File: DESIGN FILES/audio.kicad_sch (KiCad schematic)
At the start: 22 parts, among them J501 PJ-342B-TX-SMT, J502 PJ-342B-TX-SMT, J503 PJ-342B-TX-SMT, U501 WM8978CGEFL_RV

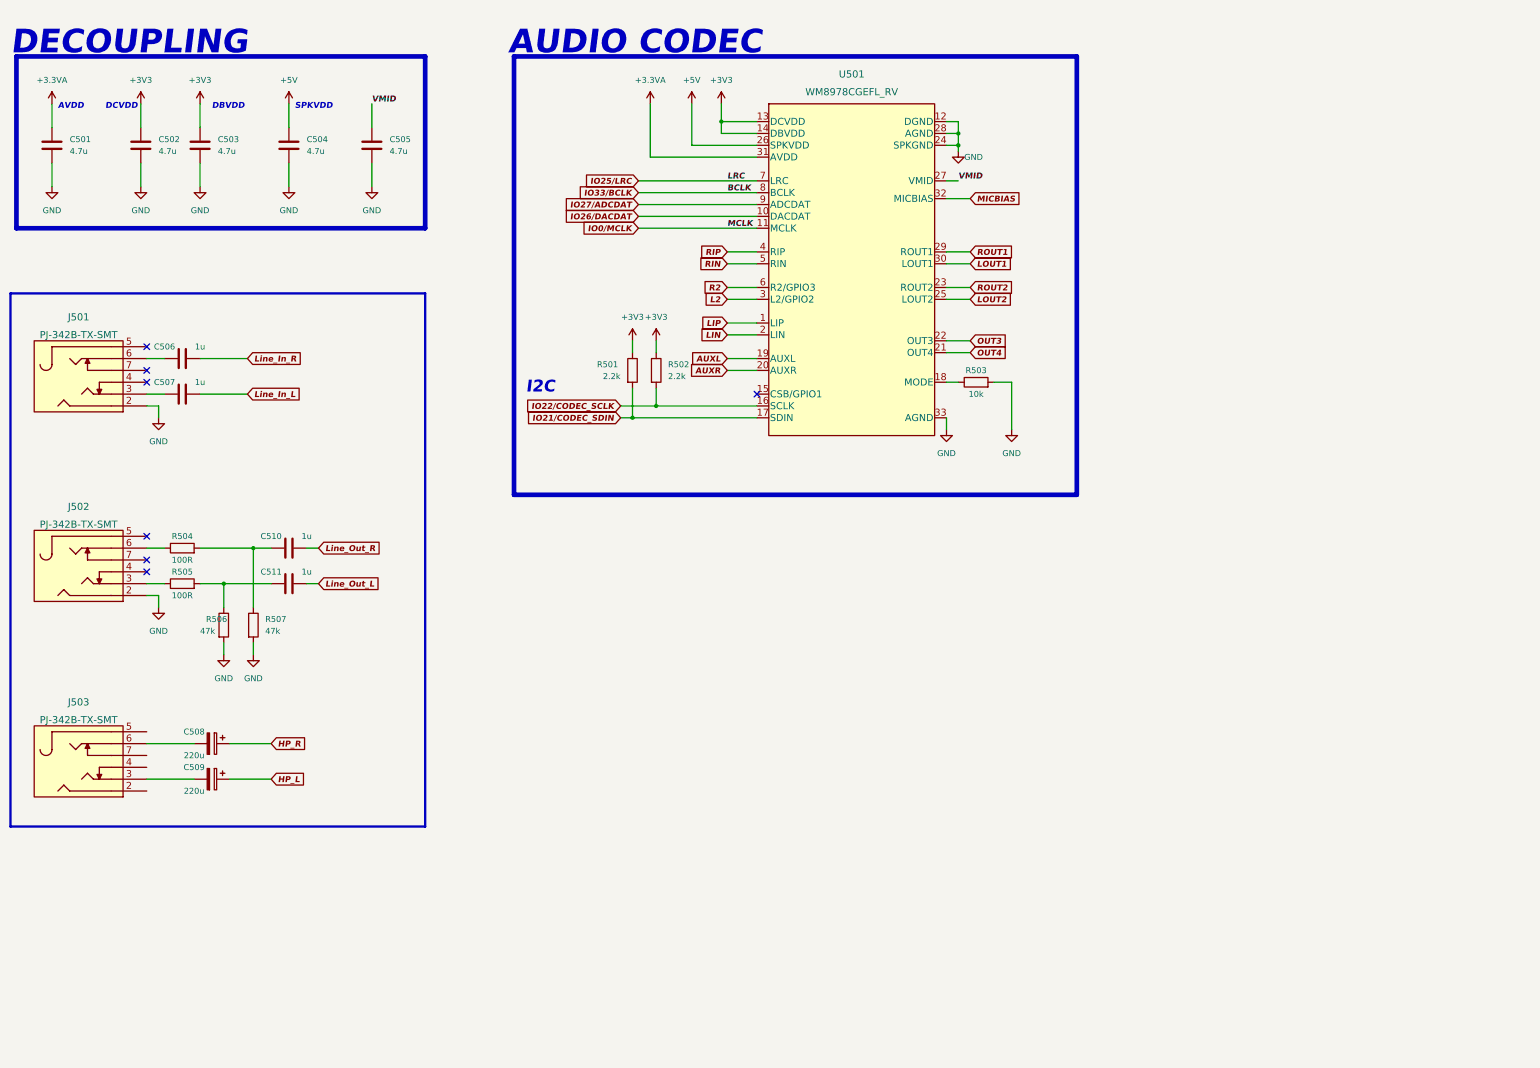
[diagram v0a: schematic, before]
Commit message: updates
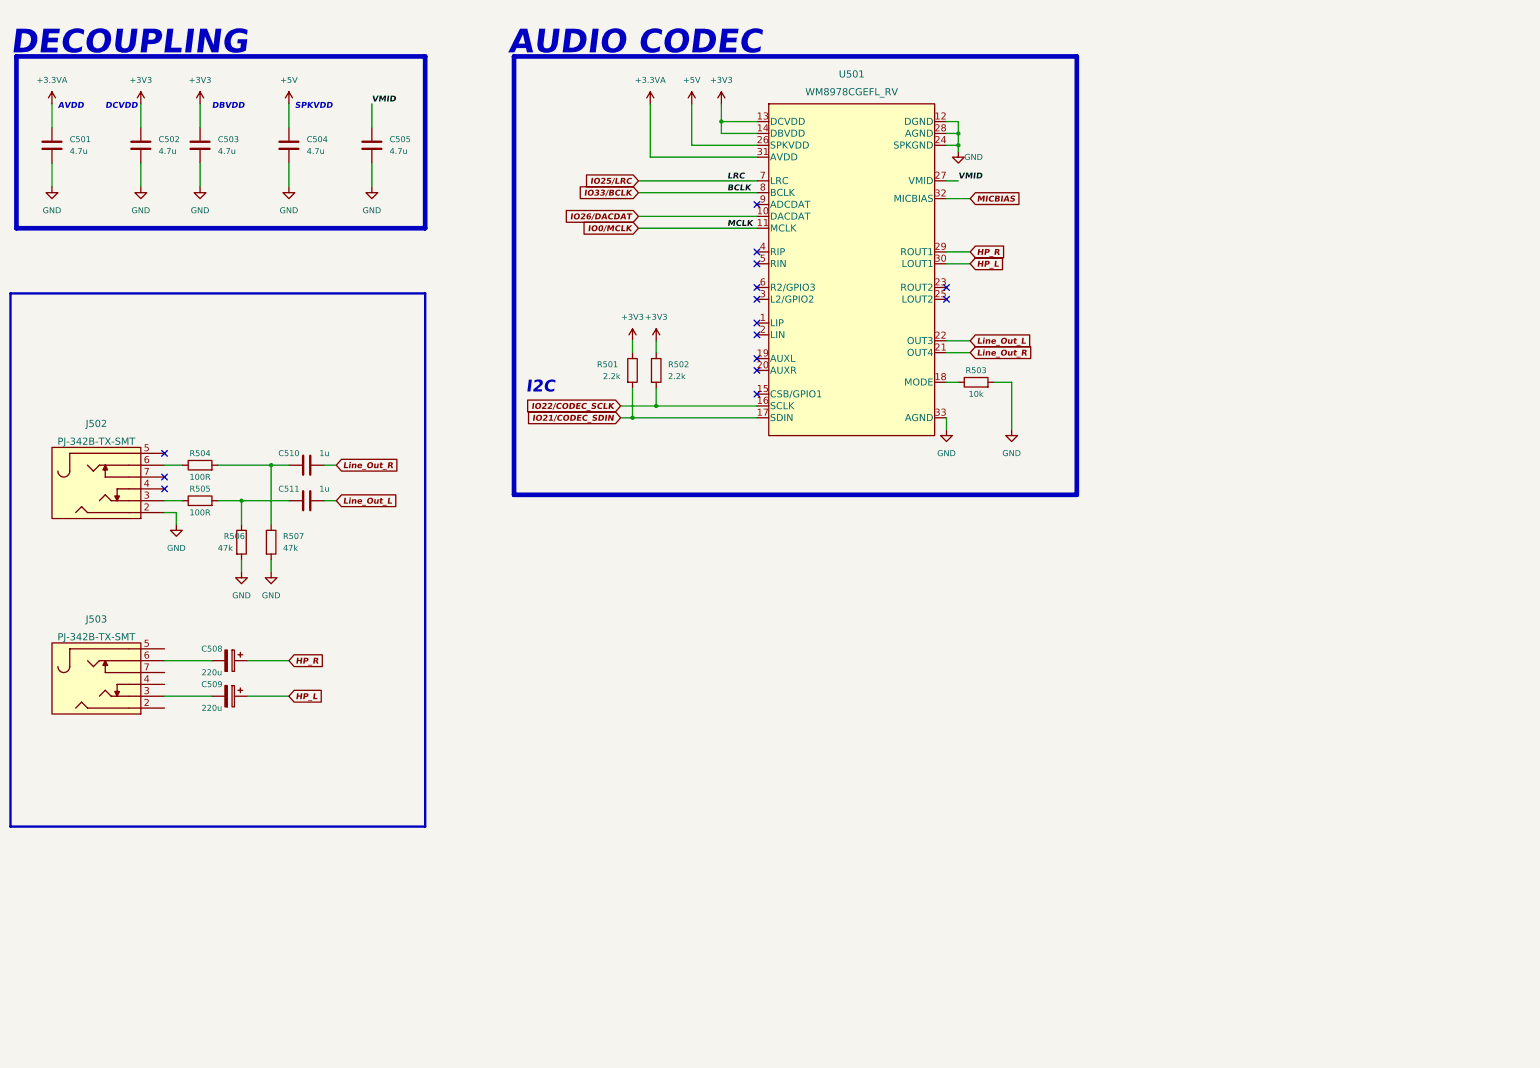
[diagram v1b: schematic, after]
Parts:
- removed C506, C507: 1u, MY CAPACITOR LIBRARY:CL10A105KB8NNNC_0603, symbol MY CAPACITOR LIBRARY:CL10A105KB8NNNC
- removed J501: PJ-342B-TX-SMT, MY CONNECTOR LIBRARY:PJ-342B-TX-SMT, symbol MY CONNECTOR LIBRARY:PJ-342B-TX-SMT
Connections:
- net LOUT1 is gone; now on net HP_L: U501.30 (LOUT1)
- net OUT3 is gone; now on net Line_Out_L: U501.22 (OUT3)
- net OUT4 is gone; now on net Line_Out_R: U501.21 (OUT4)
- net ROUT1 is gone; now on net HP_R: U501.29 (ROUT1)
- net AUXL: no longer names the net of U501.19 (AUXL)
- net AUXR: no longer names the net of U501.20 (AUXR)
- net IO27/ADCDAT: no longer names the net of U501.9 (ADCDAT)
- net L2: no longer names the net of U501.3 (L2/GPIO2)
- net LIN: no longer names the net of U501.2 (LIN)
- net LIP: no longer names the net of U501.1 (LIP)
- net LOUT2: no longer names the net of U501.25 (LOUT2)
- net R2: no longer names the net of U501.6 (R2/GPIO3)
- net RIN: no longer names the net of U501.5 (RIN)
- net RIP: no longer names the net of U501.4 (RIP)
- net ROUT2: no longer names the net of U501.23 (ROUT2)
- no-connect marks 7 -> 15
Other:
- moved on the sheet: C508, C509, C510, C511, J502, J503, R504, R505, R506, R507

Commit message: updates
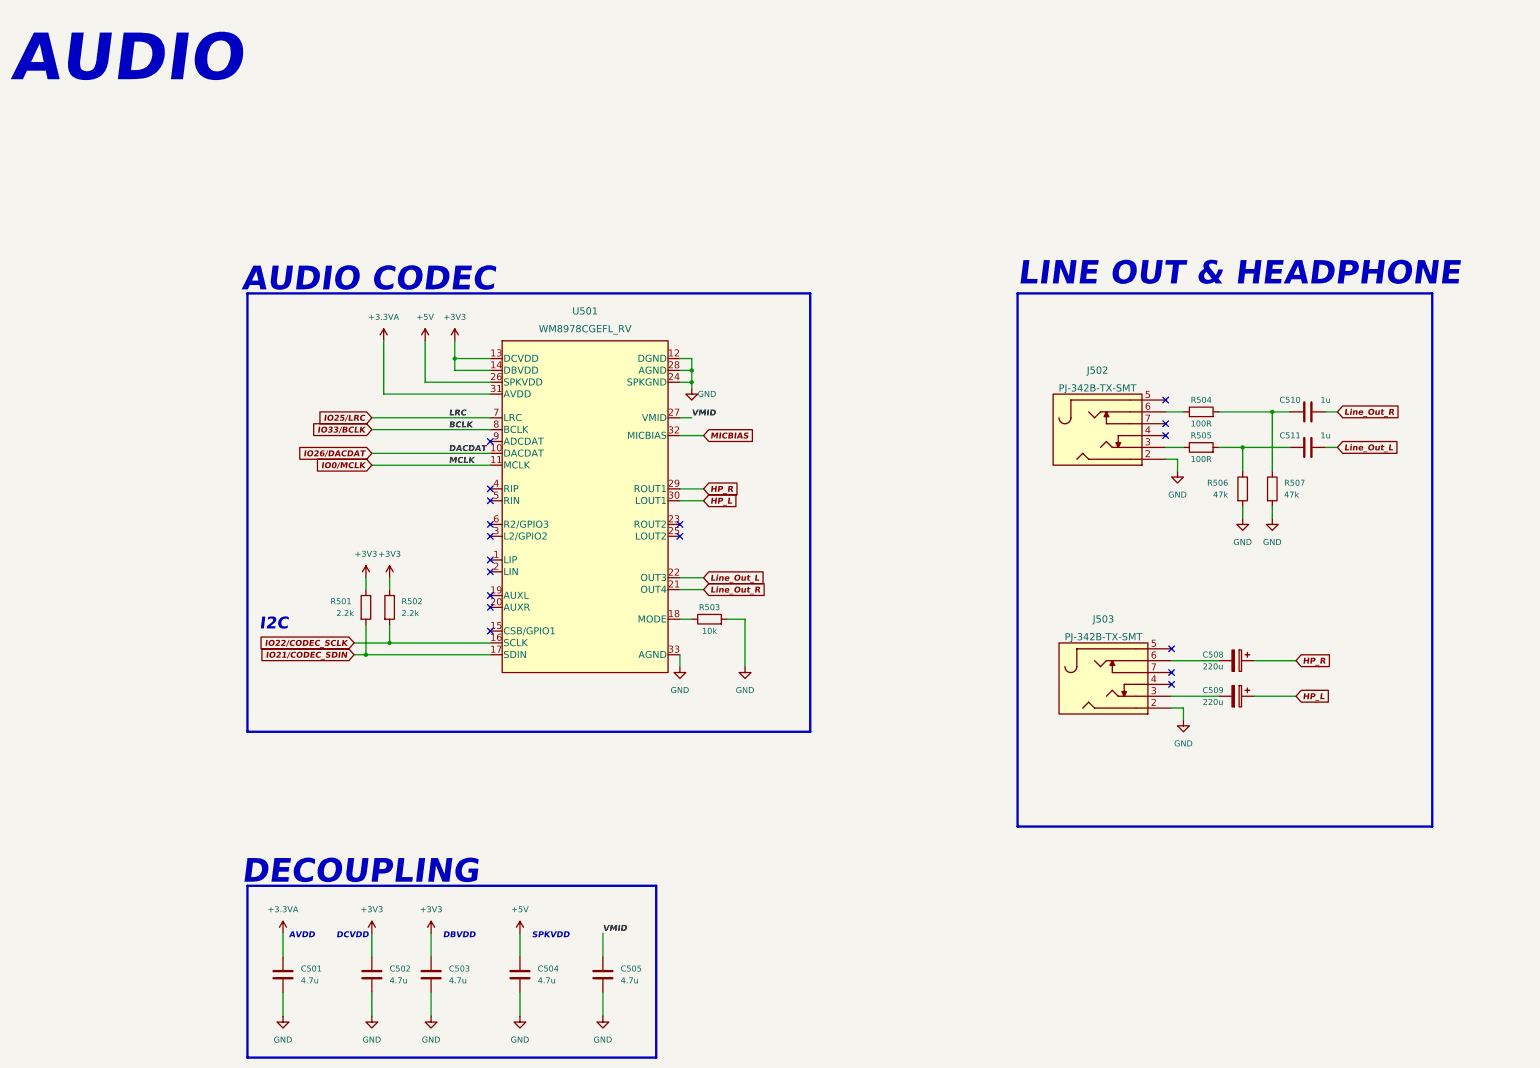
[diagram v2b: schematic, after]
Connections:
- net GND: now also J503.2
- no-connect marks 15 -> 18
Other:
- note added: "AUDIO"
- note added: "LINE OUT & HEADPHONE"
- company: (none) -> Joël Ucedo
- title: (none) -> ESP32 SYNTH
- moved on the sheet: C501, C502, C503, C504, C505, C508, C509, C510, C511, J502, J503, R501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
